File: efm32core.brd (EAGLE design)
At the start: 52.1 x 53.3 mm, 37 parts, among them U1 IP4220CZ6SSOT-6

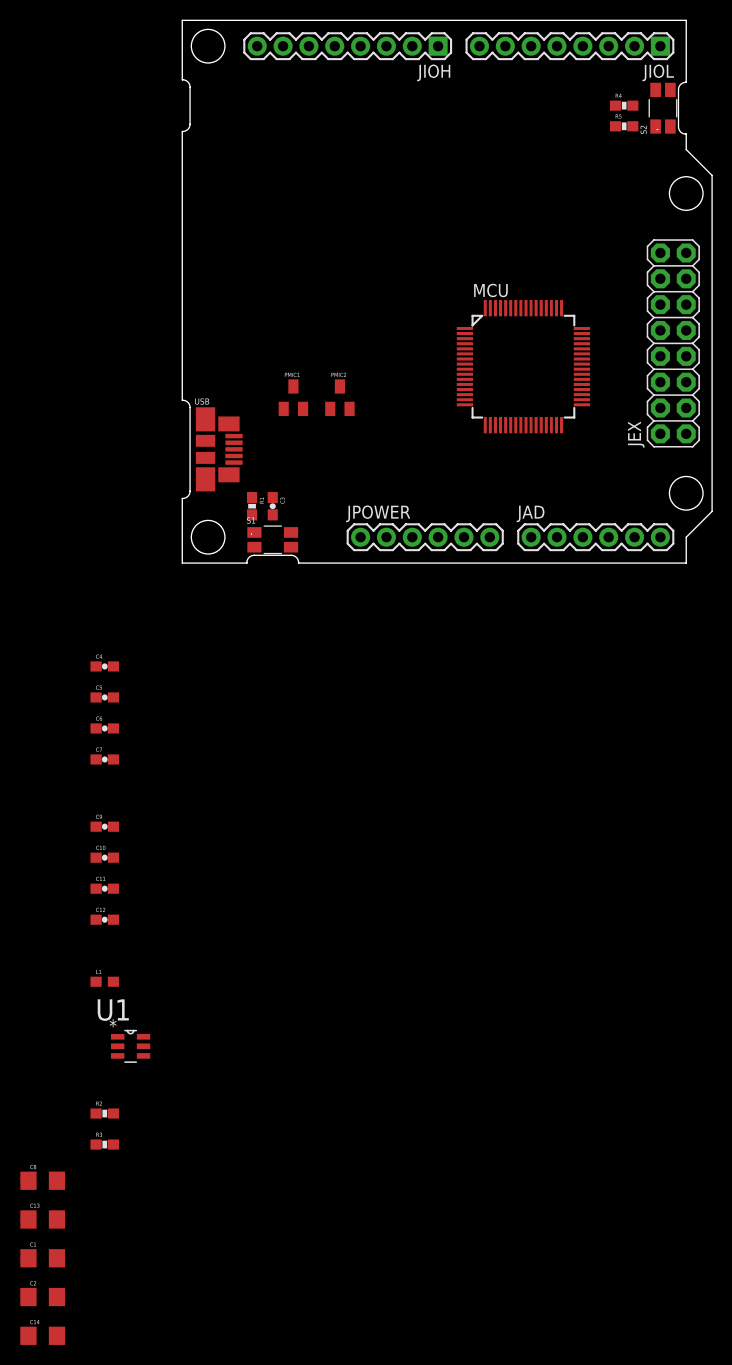
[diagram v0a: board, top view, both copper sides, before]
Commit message: layout components
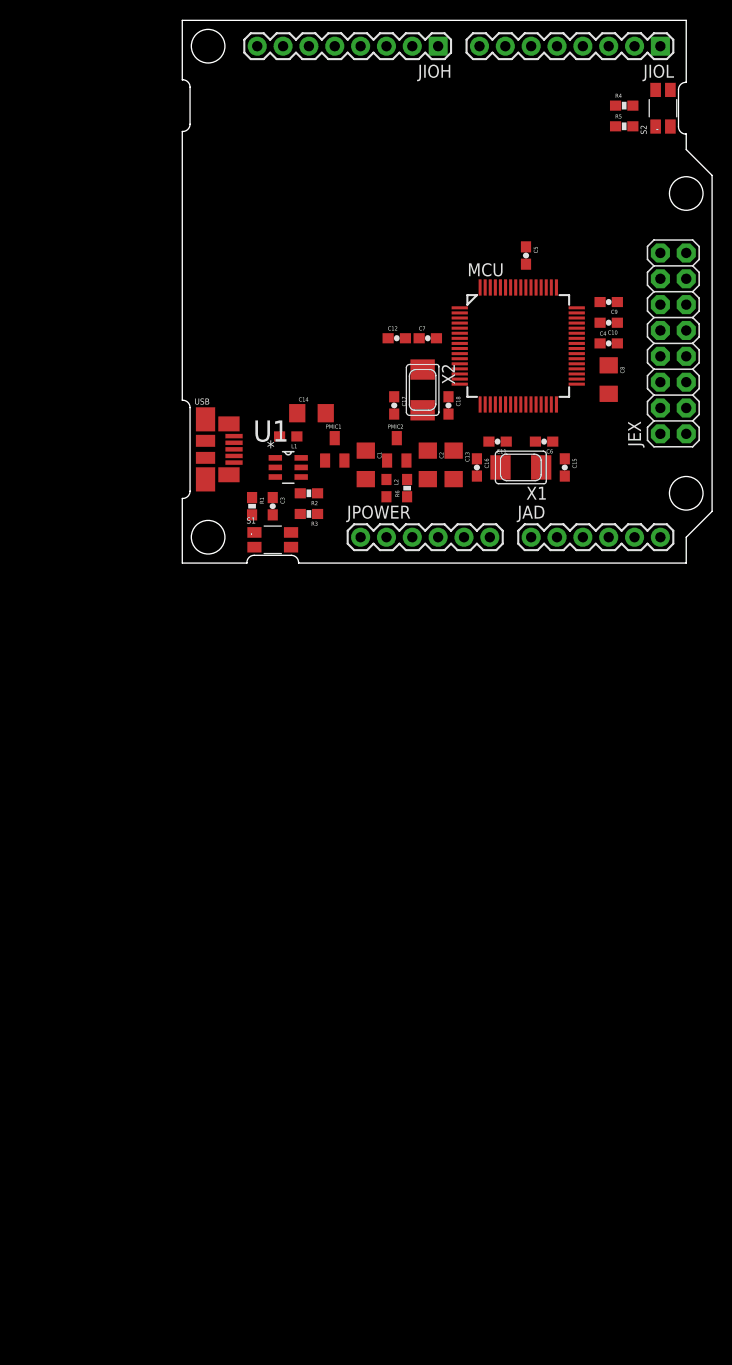
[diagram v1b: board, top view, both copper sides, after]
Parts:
- added C15, C16: 7p5, SparkFun-Capacitors:0603-CAP
- added C17, C18: 18p, SparkFun-Capacitors:0603-CAP
- added L2: (no value), SparkFun-Passives:0603
- added R6: 100, SparkFun-Resistors:0603-RES
- added X1: 48.0MHz, adafruit:NX5032
- added X2: 32.768kHz, adafruit:NX5032
- moved C8 96.4 mm to (41.9, 18.0), turned to 270 degrees
- moved C14 94.4 mm to (12.7, 14.7)
- moved C2 90.1 mm to (24.1, 9.65), turned to 270 degrees
- moved C13 84.5 mm to (26.7, 9.65), turned to 270 degrees
- moved C1 84.2 mm to (18.0, 9.65), turned to 270 degrees
- moved C10 72.2 mm to (41.9, 23.6), turned to 180 degrees
- moved C9 71.5 mm to (41.9, 25.7), turned to 180 degrees
- moved R3 65.1 mm to (12.4, 4.83), turned to 180 degrees
- moved R2 64.2 mm to (12.4, 6.86), turned to 180 degrees
- moved C12 64.0 mm to (21.1, 22.1)
- moved C5 60.0 mm to (33.8, 30.2), turned to 270 degrees
- moved U1 59.0 mm to (10.4, 9.40)
- moved C4 58.8 mm to (41.9, 21.6)
- moved C11 58.5 mm to (31.0, 11.9), turned to 180 degrees
- moved L1 56.5 mm to (10.4, 12.4), turned to 180 degrees
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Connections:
- removed net N$10: C11.1, C12.1, C13.1, MCU.23, MCU.27
- new net HFXTAL_N: C15.1, MCU.25, X1.P$2
- new net HFXTAL_P: C16.1, MCU.24, X1.P$1
- new net LFXTAL_N: C18.1, MCU.16, X2.P$1
- new net LFXTAL_P: C17.1, MCU.15, X2.P$2
- new net N$4: L2.2, R6.1
- new net N$9: R5.1, S2.B3
- new net PA0: MCU.1
- net 3.3V: now also C5.2, C6.2, C7.2, C8.2, L2.1, MCU.26, MCU.39, MCU.55, MCU.7
- net 5V: no longer C5.2, C6.2, C7.2, C8.2, MCU.26, MCU.39, MCU.55, MCU.7
- net GND: now also C15.2, C16.2, C17.2, C18.2
- net VDD: now also C11.1, C12.1, C13.1, MCU.23, MCU.27, R6.2
